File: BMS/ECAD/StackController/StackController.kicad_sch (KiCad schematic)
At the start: 10 parts, among them U1 TLE9012, U2 TMUX1309A, U3 TMUX1309A

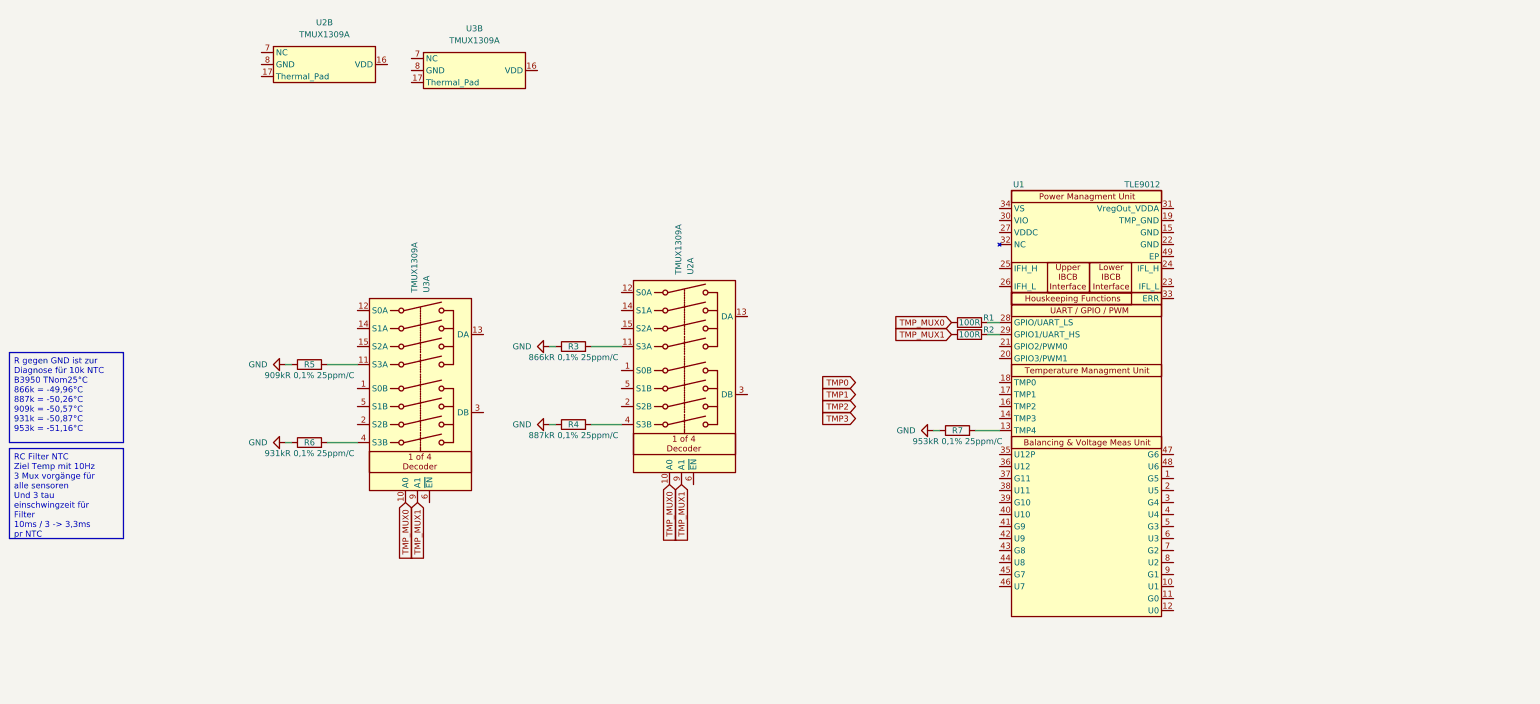
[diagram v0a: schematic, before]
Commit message: started stack controller design
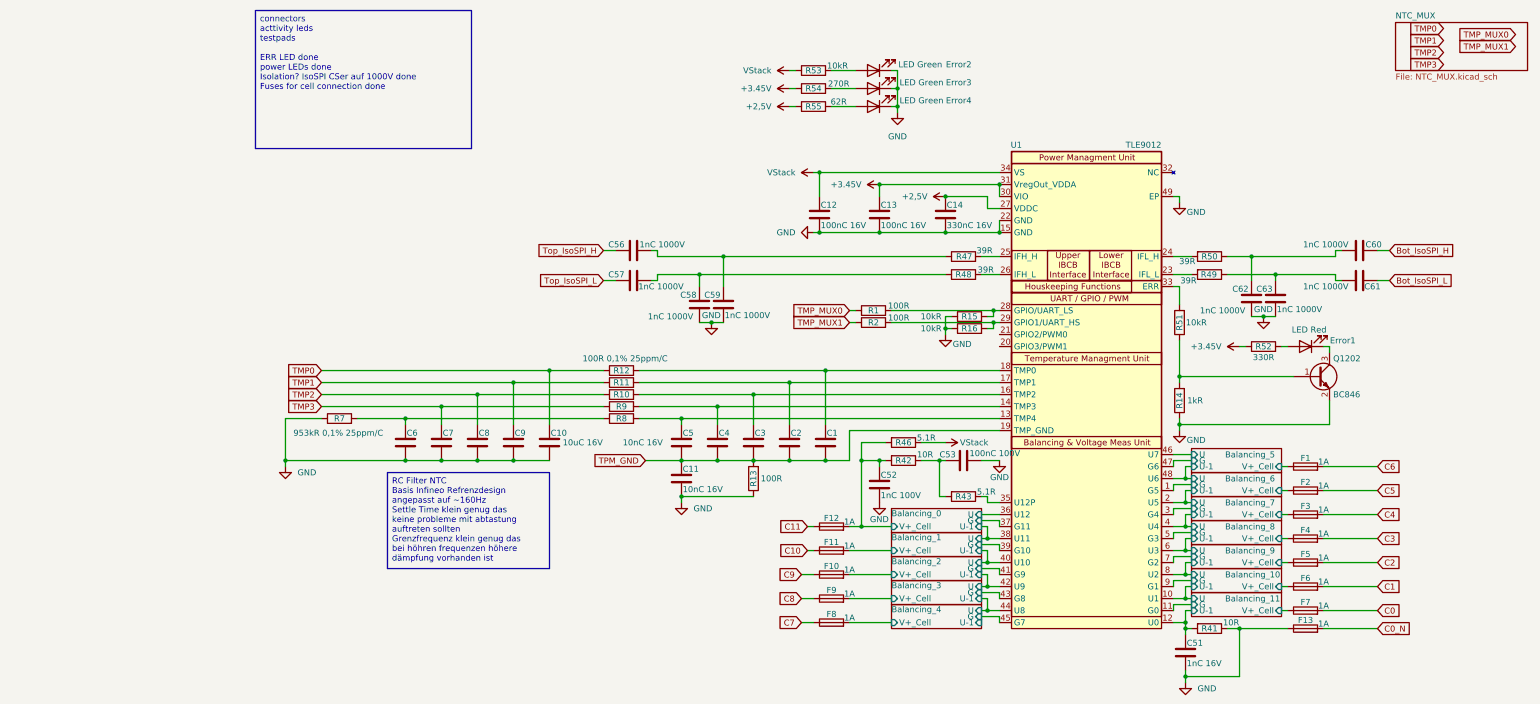
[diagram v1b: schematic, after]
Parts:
- removed R3: 866kR 0,1% 25ppm/C, Resistor_SMD:R_0603_1608Metric, symbol Device:R
- removed R4: 887kR 0,1% 25ppm/C, Resistor_SMD:R_0603_1608Metric, symbol Device:R
- removed R5: 909kR 0,1% 25ppm/C, Resistor_SMD:R_0603_1608Metric, symbol Device:R
- removed R6: 931kR 0,1% 25ppm/C, Resistor_SMD:R_0603_1608Metric, symbol Device:R
- removed U2, U3: TMUX1309A, symbol EKartParts:TMUX1309A
- added C1, C11, C2, C3, C4, C5: 10nC 16V, Capacitor_SMD:C_0603_1608Metric, symbol Device:C
- added C10: 10uC 16V, Capacitor_SMD:C_0805_2012Metric, symbol Device:C
- added C12, C13: 100nC 16V, Capacitor_SMD:C_0603_1608Metric, symbol Device:C
- added C14: 330nC 16V, Capacitor_SMD:C_0603_1608Metric, symbol Device:C
- added C51: 1nC 16V, Capacitor_SMD:C_0603_1608Metric, symbol Device:C
- added C52: 1nC 100V, Capacitor_SMD:C_0603_1608Metric, symbol Device:C
- added C53: 100nC 100V, Capacitor_SMD:C_0603_1608Metric, symbol Device:C
- added C56, C57, C58, C59, C60, C61, C62, C63: 1nC 1000V, Capacitor_SMD:C_1206_3216Metric, symbol Device:C
- added C6, C7, C8, C9: 10uC 16V, Capacitor_SMD:C_0603_1608Metric, symbol Device:C
- added Error1: LED Red, LED_SMD:LED_0805_2012Metric_Pad1.15x1.40mm_HandSolder, symbol Device:LED
- added Error2, Error3, Error4: LED Green, LED_SMD:LED_0805_2012Metric_Pad1.15x1.40mm_HandSolder, symbol Device:LED
- added F1, F10, F11, F12, F13, F2, F3, F4, F5, F6, F7, F8, F9: 1A, Fuse:Fuse_0603_1608Metric, symbol Device:Fuse
- added Q1202: BC846, Package_TO_SOT_SMD:SOT-23, symbol Transistor_BJT:BC846
- added R10, R11, R12, R8, R9: 100R 0,1% 25ppm/C, Resistor_SMD:R_0603_1608Metric, symbol Device:R
- added R13: 100R, Resistor_SMD:R_0603_1608Metric, symbol Device:R
- added R14: 1kR, Resistor_SMD:R_0603_1608Metric, symbol Device:R
- added R15, R16, R51: 10kR, Resistor_SMD:R_0603_1608Metric, symbol Device:R
- added R41, R42: 10R, Resistor_SMD:R_2512_6332Metric, symbol Device:R
- added R43, R46: 5.1R, Resistor_SMD:R_2512_6332Metric, symbol Device:R
- added R47, R48, R49, R50: 39R, Resistor_SMD:R_0603_1608Metric, symbol Device:R
- added R52: 330R, Resistor_SMD:R_0603_1608Metric, symbol Device:R
- added R53: 10kR, Resistor_SMD:R_0805_2012Metric, symbol Device:R
- added R54: 270R, Resistor_SMD:R_0603_1608Metric, symbol Device:R
- added R55: 62R, Resistor_SMD:R_0603_1608Metric, symbol Device:R
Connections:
- net GND: now also U1.15 (GND), U1.22 (GND), U1.49 (EP), C10.2, C11.2, C12.2, C13.2, C14.2, C51.2, C52.2, C53.1, C58.2, C59.2, C6.2, C62.2, C63.2, C7.2, C8.2, C9.2, Error2.1 (K), Error3.1 (K), Error4.1 (K), F13.1, Q1202.2 (E), R13.1, R14.1, R15.1, R16.1, R41.1
- net TMP0: now also C10.1, R12.1
- net TMP1: now also C9.1, R11.1
- net TMP2: now also C8.1, R10.1
- net TMP3: now also C7.1, R9.1
- net at R1.2, U1.28 (GPIO/UART_LS): now also R15.2
- net at R2.2, U1.29 (GPIO1/UART_HS): now also R16.2
- net Balancing_6/G: now reaches U1.1 (G5)
- net Balancing_10/U-1: now reaches U1.10 (U1)
- net Balancing_11/G: now reaches U1.11 (G0)
- net Balancing_11/U-1: now reaches U1.12 (U0)
- net Balancing_11/U-1: now also C51.1, R41.2
- net at U1.13 (TMP4): now also C5.1, R8.2; no longer R7.2
- net at U1.14 (TMP3): now also C4.1, R9.2
- net at U1.16 (TMP2): now also C3.1, R10.2
- net at U1.17 (TMP1): now also C2.1, R11.2
- net at U1.18 (TMP0): now also C1.1, R12.2
- net TPM_GND: now reaches U1.19 (TMP_GND)
- net TPM_GND: now also C1.2, C11.1, C2.2, C3.2, C4.2, C5.2, R13.2
- net Balancing_6/U-1: now reaches U1.2 (U5)
- net at U1.23 (IFL_L): now also R49.2
- net at U1.24 (IFL_H): now also R50.2
- net at U1.25 (IFH_H): now also R47.2
- net at U1.26 (IFH_L): now also R48.2
- net +2,5V: now reaches U1.27 (VDDC)
- net +2,5V: now also C14.1, R55.1
- net Balancing_7/G: now reaches U1.3 (G4)
- net +3.45V: now reaches U1.30 (VIO)
- net +3.45V: now also U1.31 (VregOut_VDDA), C13.1, R52.1, R54.1
- net at U1.33 (ERR): now also R51.2
- net VStack: now reaches U1.34 (VS)
- net VStack: now also C12.1, R46.1, R53.1
- net at U1.35 (U12P): now also R43.1
- net Balancing_0/U: now reaches U1.36 (U12)
- net Balancing_0/G: now reaches U1.37 (G11)
- net Balancing_0/U-1: now reaches U1.38 (U11)
- net Balancing_1/G: now reaches U1.39 (G10)
- net Balancing_7/U-1: now reaches U1.4 (U4)
- net Balancing_1/U-1: now reaches U1.40 (U10)
- net Balancing_2/G: now reaches U1.41 (G9)
- net Balancing_2/U-1: now reaches U1.42 (U9)
- net Balancing_3/G: now reaches U1.43 (G8)
- net Balancing_3/U-1: now reaches U1.44 (U8)
- net Balancing_4/G: now reaches U1.45 (G7)
- net Balancing_5/U: now reaches U1.46 (U7)
- net Balancing_5/G: now reaches U1.47 (G6)
- net Balancing_5/U-1: now reaches U1.48 (U6)
- net Balancing_8/G: now reaches U1.5 (G3)
- net Balancing_8/U-1: now reaches U1.6 (U3)
- net Balancing_9/G: now reaches U1.7 (G2)
- net Balancing_10/U: now reaches U1.8 (U2)
- net Balancing_10/G: now reaches U1.9 (G1)
- new net: C61.2, C63.1, R49.1
- new net: C57.1, C58.1, R48.1
- new net: Q1202.1 (B), R14.2, R51.1
- new net: Error1.1 (K), Q1202.3 (C)
- new net: Error1.2 (A), R52.2
- new net: C6.1, R7.2, R8.1
- new net: Error3.2 (A), R54.2
- new net: Error4.2 (A), R55.2
- new net: C53.2, R42.1, R43.2
- new net: Error2.2 (A), R53.2
- new net: C60.2, C62.1, R50.1
- new net: C56.1, C59.1, R47.1
- new net Balancing_0/V+_Cell: C52.1, F12.2, R42.2, R46.2
- new net Balancing_1/V+_Cell: F11.2
- new net Balancing_10/V+_Cell: F6.1
- new net Balancing_11/V+_Cell: F7.1
- new net Balancing_2/V+_Cell: F10.2
- new net Balancing_3/V+_Cell: F9.2
- new net Balancing_4/V+_Cell: F8.2
- new net Balancing_5/V+_Cell: F1.1
- new net Balancing_6/V+_Cell: F2.1
- new net Balancing_7/V+_Cell: F3.1
- new net Balancing_8/V+_Cell: F4.1
- new net Balancing_9/V+_Cell: F5.1
- new net Bot_IsoSPI_H: C60.1
- new net Bot_IsoSPI_L: C61.1
- new net C0: F7.2
- new net C0_N: F13.2
- new net C1: F6.2
- new net C10: F11.1
- new net C11: F12.1
- new net C2: F5.2
- new net C3: F4.2
- new net C4: F3.2
- new net C5: F2.2
- new net C6: F1.2
- new net C7: F8.1
- new net C8: F9.1
- new net C9: F10.1
- new net Top_IsoSPI_H: C56.2
- new net Top_IsoSPI_L: C57.2
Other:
- added sheet Balancing_0 (Balancing.kicad_sch)
- added sheet Balancing_1 (Balancing.kicad_sch)
- added sheet Balancing_10 (Balancing.kicad_sch)
- added sheet Balancing_11 (Balancing.kicad_sch)
- added sheet Balancing_2 (Balancing.kicad_sch)
- added sheet Balancing_3 (Balancing.kicad_sch)
- added sheet Balancing_4 (Balancing.kicad_sch)
- added sheet Balancing_5 (Balancing.kicad_sch)
- added sheet Balancing_6 (Balancing.kicad_sch)
- added sheet Balancing_7 (Balancing.kicad_sch)
- added sheet Balancing_8 (Balancing.kicad_sch)
- added sheet Balancing_9 (Balancing.kicad_sch)
- added sheet NTC_MUX (NTC_MUX.kicad_sch)
- moved on the sheet: R1, R2, R7
